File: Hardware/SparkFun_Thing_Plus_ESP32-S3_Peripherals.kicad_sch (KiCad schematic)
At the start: 24 parts, among them J3 PH-2AWT, U1 RT9080-3.3, U4 MAX17048, U5 MCP73831, U7 TP4056-42-ESOP8, X1 C32346

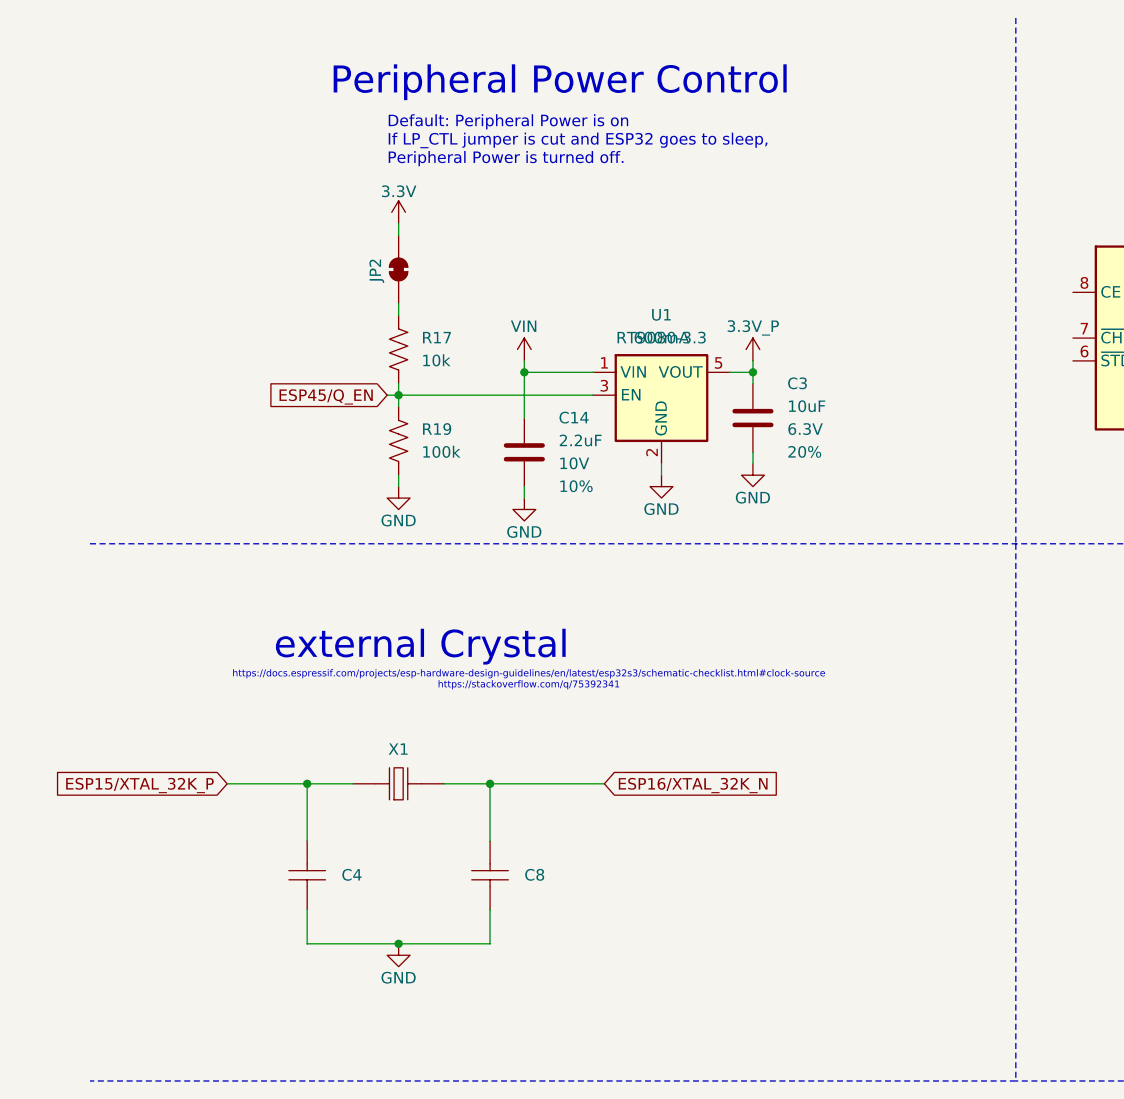
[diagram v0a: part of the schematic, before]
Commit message: temp
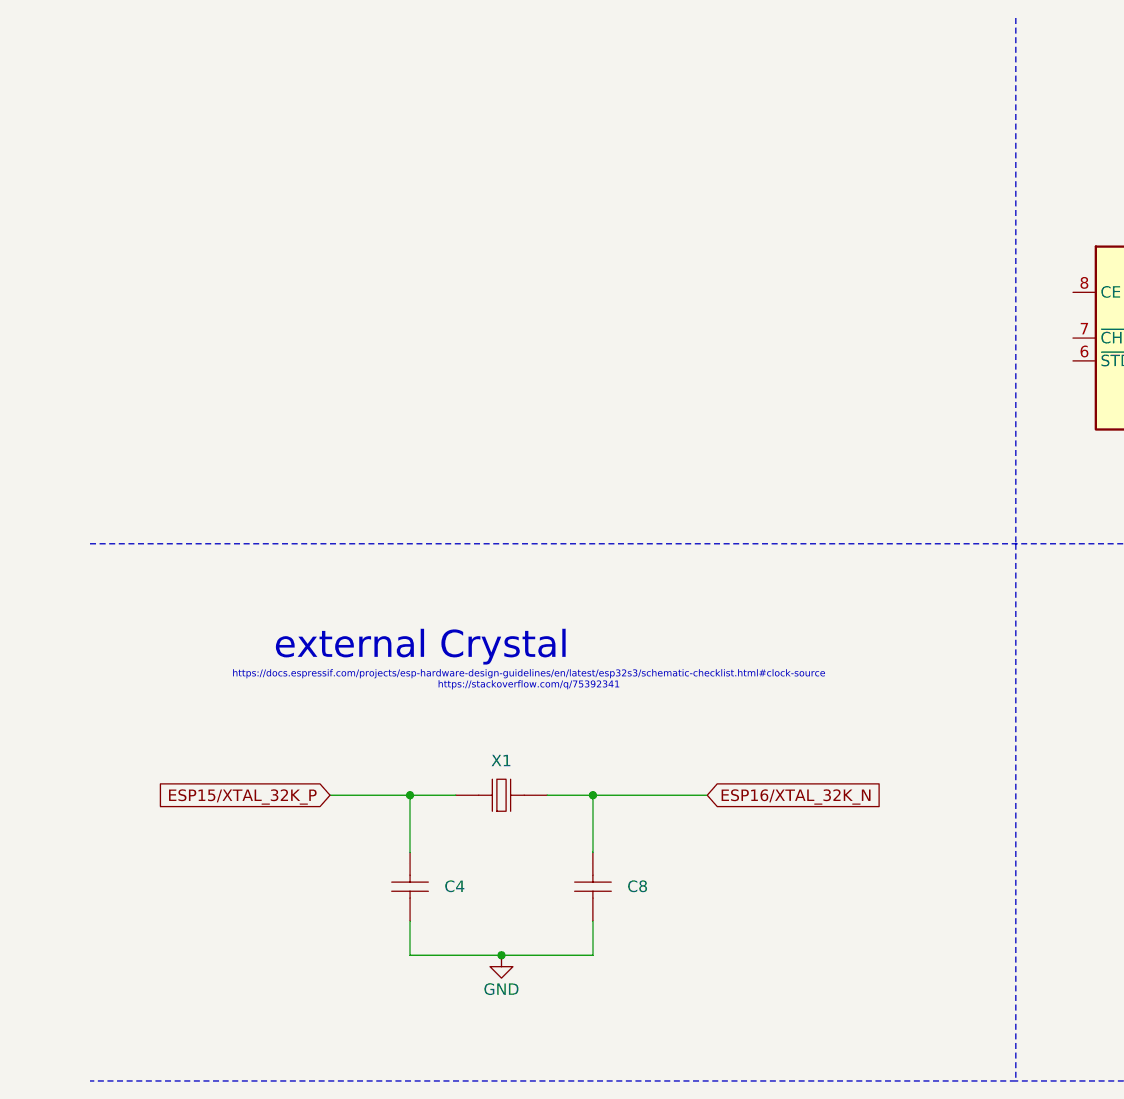
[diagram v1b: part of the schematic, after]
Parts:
- removed C14: 2.2uF, PCM_SparkFun-Capacitor:C_0402_1005Metric, symbol SparkFun-Capacitor:2.2uF_0402_10V_10%
- removed C3: 10uF, PCM_SparkFun-Capacitor:C_0402_1005Metric, symbol SparkFun-Capacitor:10uF_0402_6.3V_20%
- removed JP2: ~, Jumper:SolderJumper-2_P1.3mm_Bridged_RoundedPad1.0x1.5mm, symbol SparkFun-Jumper:SolderJumper_2_Bridged
- removed R17: 10k, Resistor_SMD:R_0402_1005Metric, symbol SparkFun-Resistor:10k_0402
- removed R19: 100k, Resistor_SMD:R_0402_1005Metric, symbol SparkFun-Resistor:100k_0402
- removed U1: RT9080-3.3, Package_TO_SOT_SMD:SOT-23-5, symbol SparkFun-Regulator:RT9080-3.3
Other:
- note removed: "Default: Peripheral Power is on If LP_CTL jumper is cut and ESP32 goes to sleep, Peripheral Power is turned off."
- note removed: "Peripheral Power Control"
- moved on the sheet: C4, C8, X1

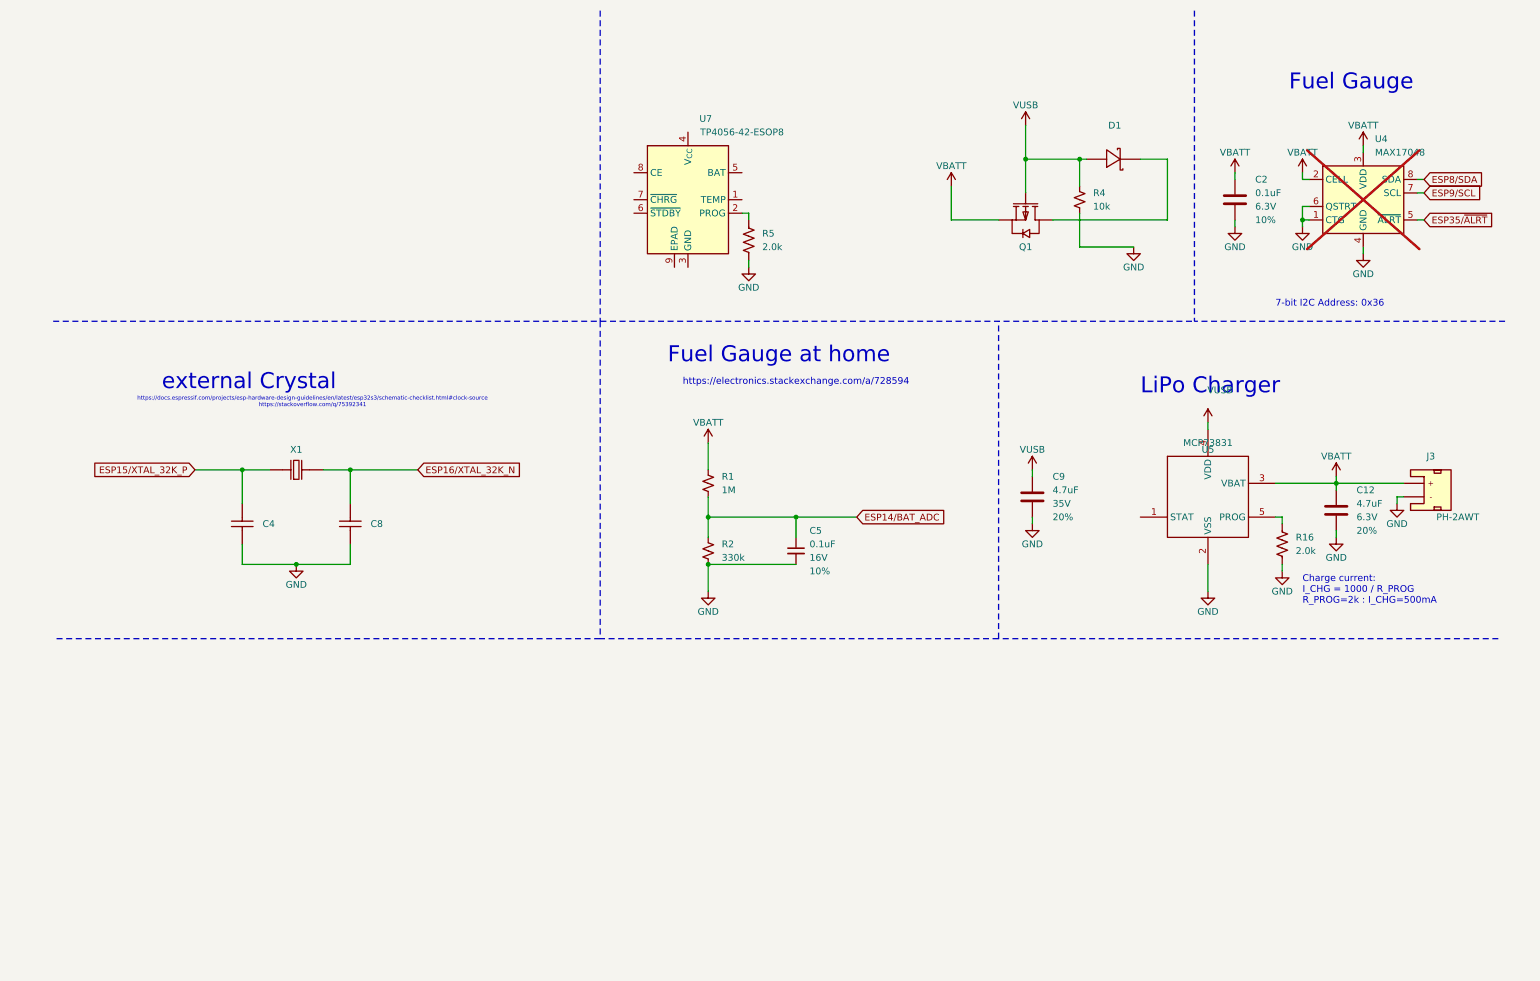
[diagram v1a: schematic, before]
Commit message: update schematic (hopefully final)
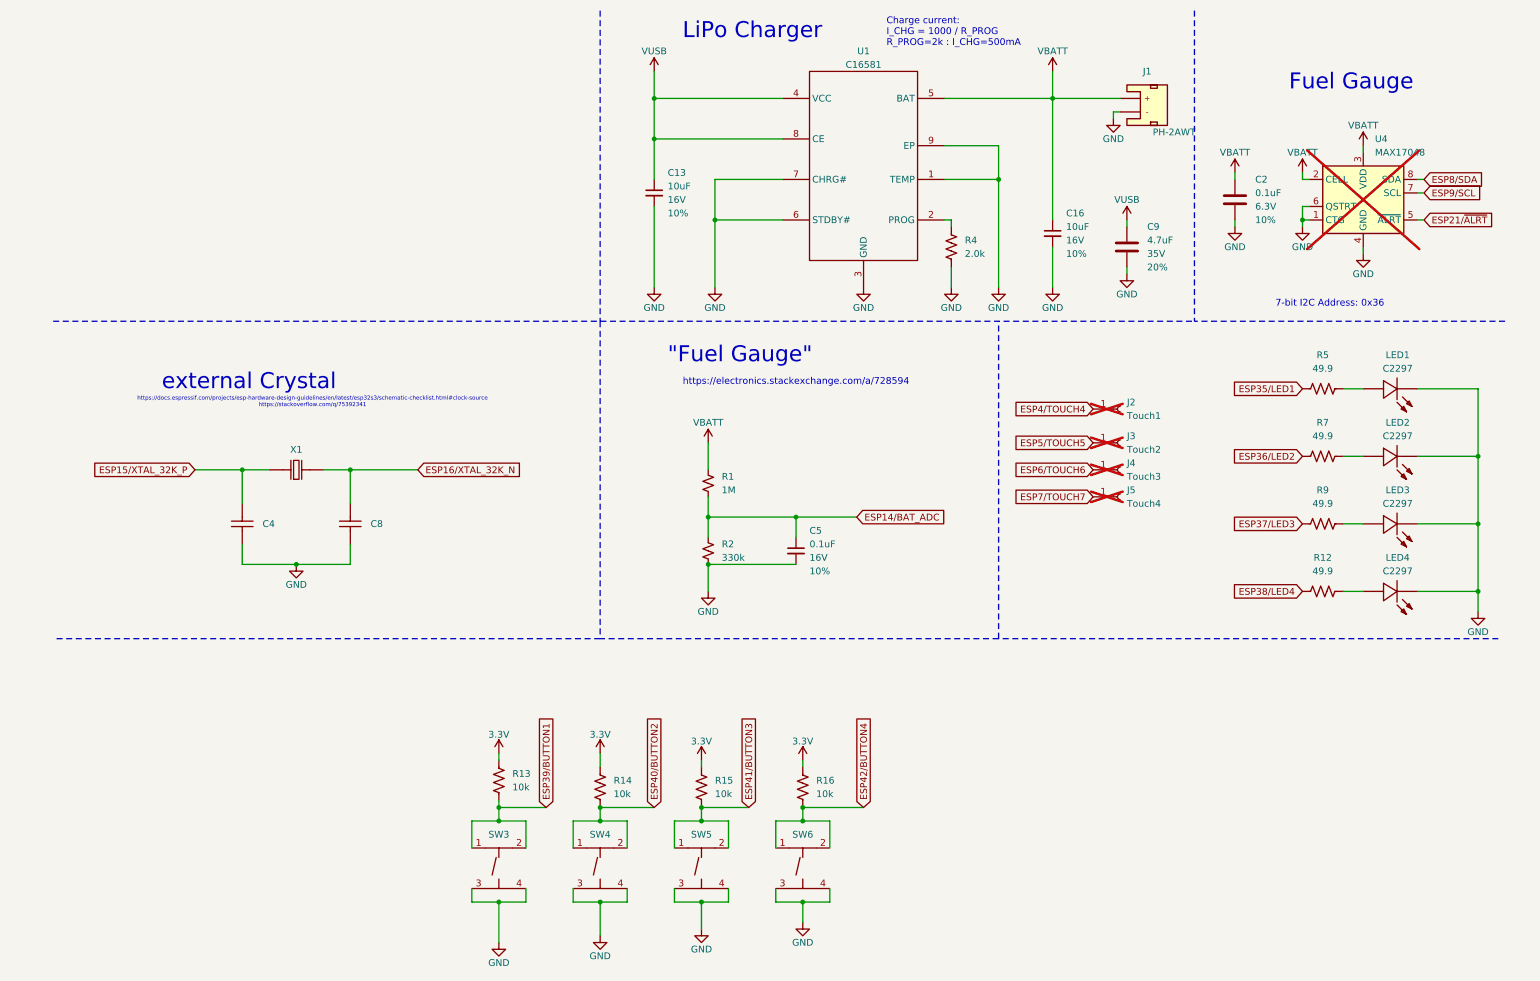
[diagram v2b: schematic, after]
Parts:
- removed C12: 4.7uF, PCM_SparkFun-Capacitor:C_0402_1005Metric, symbol SparkFun-Capacitor:4.7uF_0402_6.3V_10%
- removed D1: ~, EasyEDA_Lib:SMA_L4.3-W2.6-LS5.2-RD, symbol EasyEDA_Lib:SS34_C8678
- removed J3: PH-2AWT, EasyEDA_Lib:CONN-SMD_PH-2AWT, symbol SparkFun-Connector:Conn_01x02_JST_2mm_LiPo
- removed Q1: ~, EasyEDA_Lib:SOT-23-3_L3.0-W1.7-P0.95-LS2.9-BR, symbol EasyEDA_Lib:SI2301CDS-T1-GE3
- removed R16: 2.0k, Resistor_SMD:R_0402_1005Metric, symbol SparkFun-Resistor:2.0k_0402
- removed R4: 10k, PCM_SparkFun-Resistor:R_0402_1005Metric, symbol PCM_SparkFun-Resistor:10k_0402
- removed U5: MCP73831, EasyEDA_Lib:SOT-23-5_L3.0-W1.7-P0.95-LS2.8-BR, symbol EasyEDA_Lib:MCP73831T-2ATI/OT
- removed U7: TP4056-42-ESOP8, Package_SO:SOIC-8-1EP_3.9x4.9mm_P1.27mm_EP2.41x3.3mm_ThermalVias, symbol Battery_Management:TP4056-42-ESOP8
- added C13, C16: 10uF, PCM_SparkFun-Capacitor:C_0402_1005Metric, symbol PCM_SparkFun-Capacitor:0.1uF_0402_16V_10%
- added J1: PH-2AWT, EasyEDA_Lib:CONN-SMD_PH-2AWT, symbol SparkFun-Connector:Conn_01x02_JST_2mm_LiPo
- added J2: Touch1, symbol Connector:Conn_01x01_Socket
- added J3: Touch2, symbol Connector:Conn_01x01_Socket
- added J4: Touch3, symbol Connector:Conn_01x01_Socket
- added J5: Touch4, symbol Connector:Conn_01x01_Socket
- added LED1, LED2, LED3, LED4: C2297, EasyEDA_Lib:LED0805-R-RD, symbol EasyEDA_Lib:0805G (Green)
- added R12, R7, R9: 49.9, Resistor_SMD:R_0402_1005Metric, symbol SparkFun-Resistor:2.0k_0402
- added R13, R14, R15, R16: 10k, Resistor_SMD:R_0402_1005Metric, symbol SparkFun-Resistor:10k_0402
- added R4: 2.0k, Resistor_SMD:R_0402_1005Metric, symbol SparkFun-Resistor:2.0k_0402
- added SW3, SW4, SW5, SW6: C318884, EasyEDA_Lib:SW-SMD_4P-L5.1-W5.1-P3.70-LS6.5-TL_H1.5, symbol EasyEDA_Lib:TS-1187A-B-A-B
- added U1: C16581, EasyEDA_Lib:ESOP-8_L4.9-W3.9-P1.27-LS6.0-BL-EP, symbol EasyEDA_Lib:TP4056
- R5: value 2.0k -> 49.9
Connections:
- net GND: now also C13.2, C16.2, J1.1 (-), LED1.2 (K), LED2.2 (K), LED3.2 (K), LED4.2 (K), R4.2, SW3.3 (C), SW3.4 (D), SW4.3 (C), SW4.4 (D), SW5.3 (C), SW5.4 (D), SW6.3 (C), SW6.4 (D), U1.1 (TEMP), U1.3 (GND), U1.6 (STDBY#), U1.7 (CHRG#), U1.9 (EP); no longer R5.2
- net VBATT: now also C16.1, J1.2 (+), U1.5 (BAT)
- net VUSB: now also C13.1, U1.4 (VCC), U1.8 (CE)
- net ESP35/LED1: now reaches R5.1
- net ESP35/~{ALRT} renamed ESP21/~{ALRT}
- new net: LED2.1 (A), R7.2
- new net: LED3.1 (A), R9.2
- new net: LED1.1 (A), R5.2
- new net: J1.NC1, J1.NC2
- new net: R4.1, U1.2 (PROG)
- new net: LED4.1 (A), R12.2
- new net 3.3V: R13.1, R14.1, R15.1, R16.1
- new net ESP36/LED2: R7.1
- new net ESP37/LED3: R9.1
- new net ESP38/LED4: R12.1
- new net ESP39/BUTTON1: R13.2, SW3.1 (A), SW3.2 (B)
- new net ESP40/BUTTON2: R14.2, SW4.1 (A), SW4.2 (B)
- new net ESP41/BUTTON3: R15.2, SW5.1 (A), SW5.2 (B)
- new net ESP42/BUTTON4: R16.2, SW6.1 (A), SW6.2 (B)
- new net ESP4/TOUCH4: J2.1 (Pin_1)
- new net ESP5/TOUCH5: J3.1 (Pin_1)
- new net ESP6/TOUCH6: J4.1 (Pin_1)
- new net ESP7/TOUCH7: J5.1 (Pin_1)
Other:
- note added: ""Fuel Gauge""
- note removed: "Fuel Gauge at home"
- moved on the sheet: C9

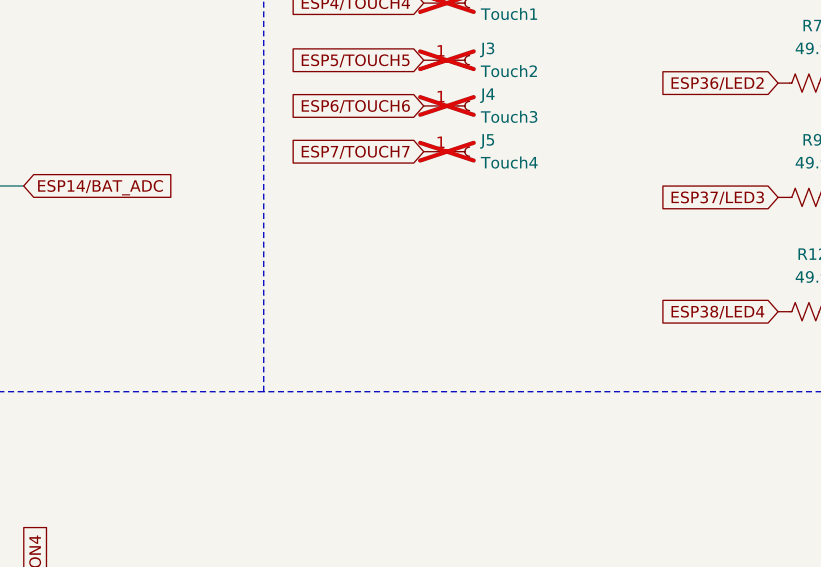
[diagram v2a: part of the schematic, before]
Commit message: .
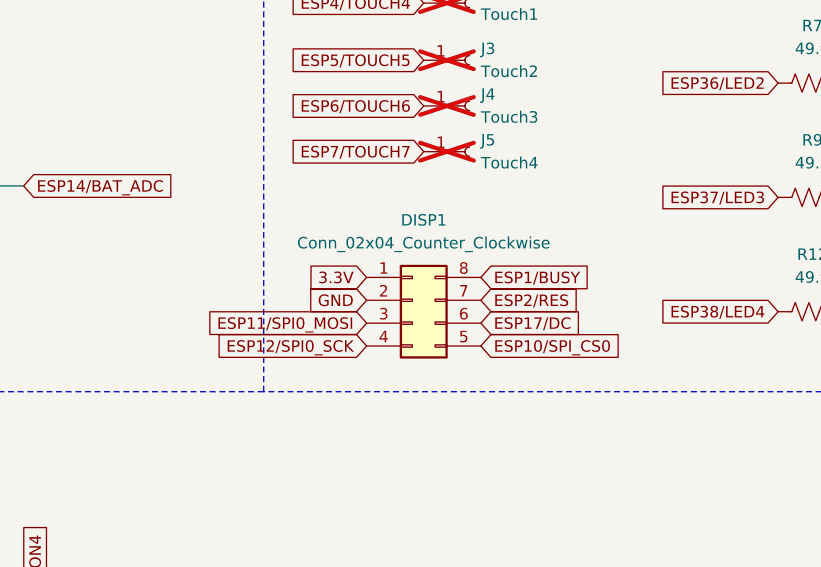
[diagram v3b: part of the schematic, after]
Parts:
- added DISP1: Conn_02x04_Counter_Clockwise, Connector_PinSocket_2.54mm:PinSocket_2x04_P2.54mm_Vertical, symbol Connector_Generic:Conn_02x04_Counter_Clockwise
- J2, J3, J4, J5: footprint (none) -> Connector_PinSocket_2.54mm:PinSocket_1x01_P2.54mm_Horizontal
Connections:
- net 3.3V: now also DISP1.1 (Pin_1)
- net GND: now also DISP1.2 (Pin_2)
- new net ESP10/SPI_CS0: DISP1.5 (Pin_5)
- new net ESP11/SPI0_MOSI: DISP1.3 (Pin_3)
- new net ESP12/SPI0_SCK: DISP1.4 (Pin_4)
- new net ESP17/DC: DISP1.6 (Pin_6)
- new net ESP1/BUSY: DISP1.8 (Pin_8)
- new net ESP2/RES: DISP1.7 (Pin_7)
